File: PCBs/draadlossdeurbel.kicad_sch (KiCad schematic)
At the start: 16 parts, among them Q1 BC161, U1 WeMos_D1_mini, U2 LM386, U3 74HC595, U4 SN76489, U5 TP4056-breakout

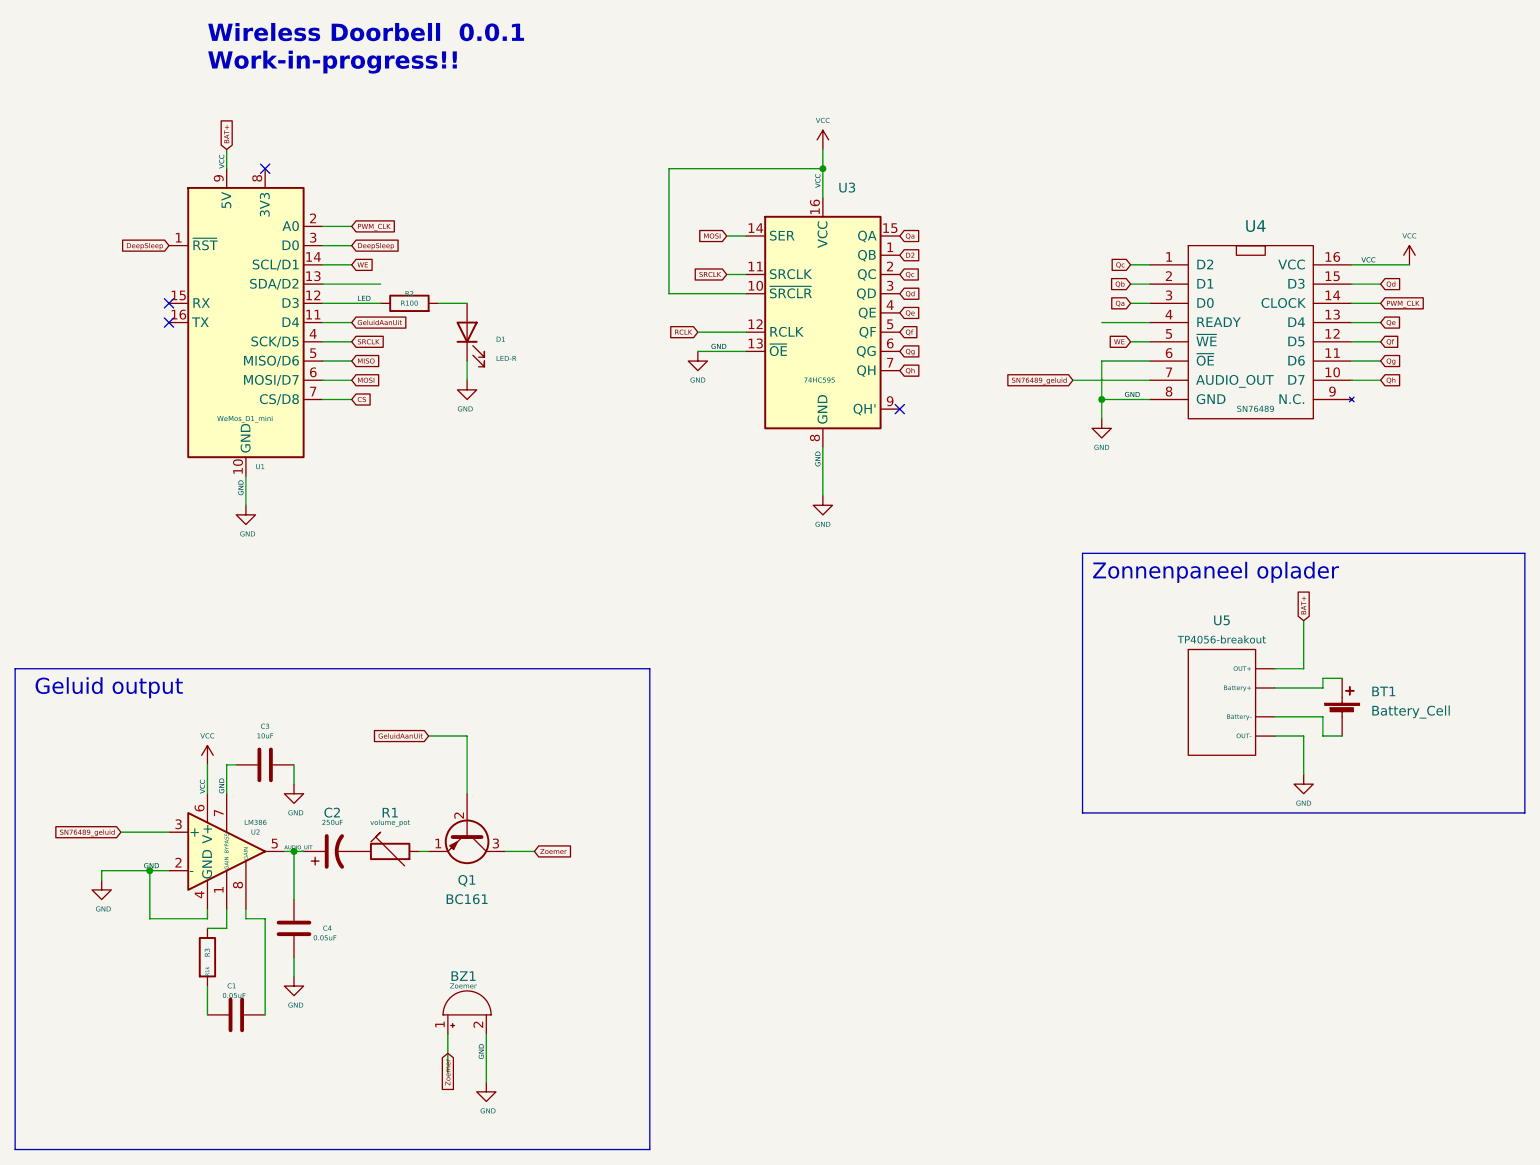
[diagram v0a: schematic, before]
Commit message: bijgewerkt
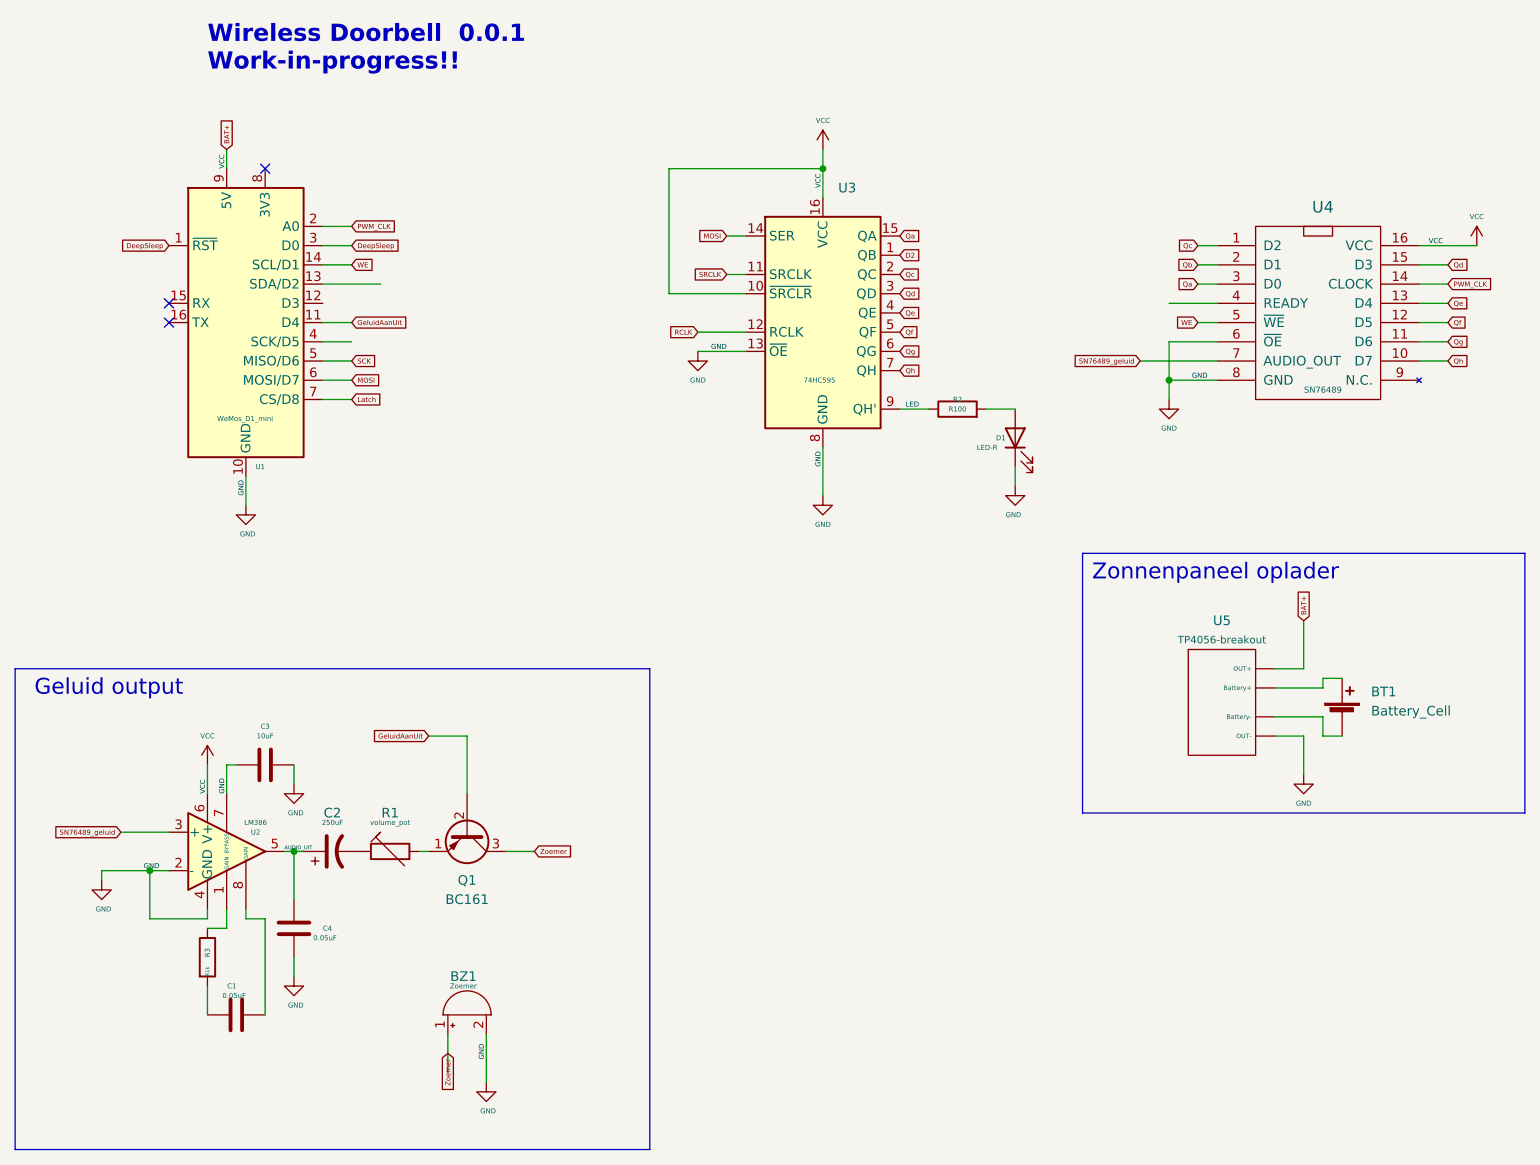
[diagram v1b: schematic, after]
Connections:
- net LED: now also U3.9 (QH'); no longer U1.12 (D3)
- net SRCLK: no longer U1.4 (SCK/D5)
- net CS renamed Latch
- net MISO renamed SCK
- no-connect marks 4 -> 3
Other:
- moved on the sheet: D1, R2, U4
